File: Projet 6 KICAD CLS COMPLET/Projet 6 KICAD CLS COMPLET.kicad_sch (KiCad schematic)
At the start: 17 parts, among them J1 Conn_02x20_Odd_Even, J2 Conn_01x06, J3 Screw_Terminal_01x04, J4 Screw_Terminal_01x04, U2 AZ1117-3.3, U3 LSM6DSOX

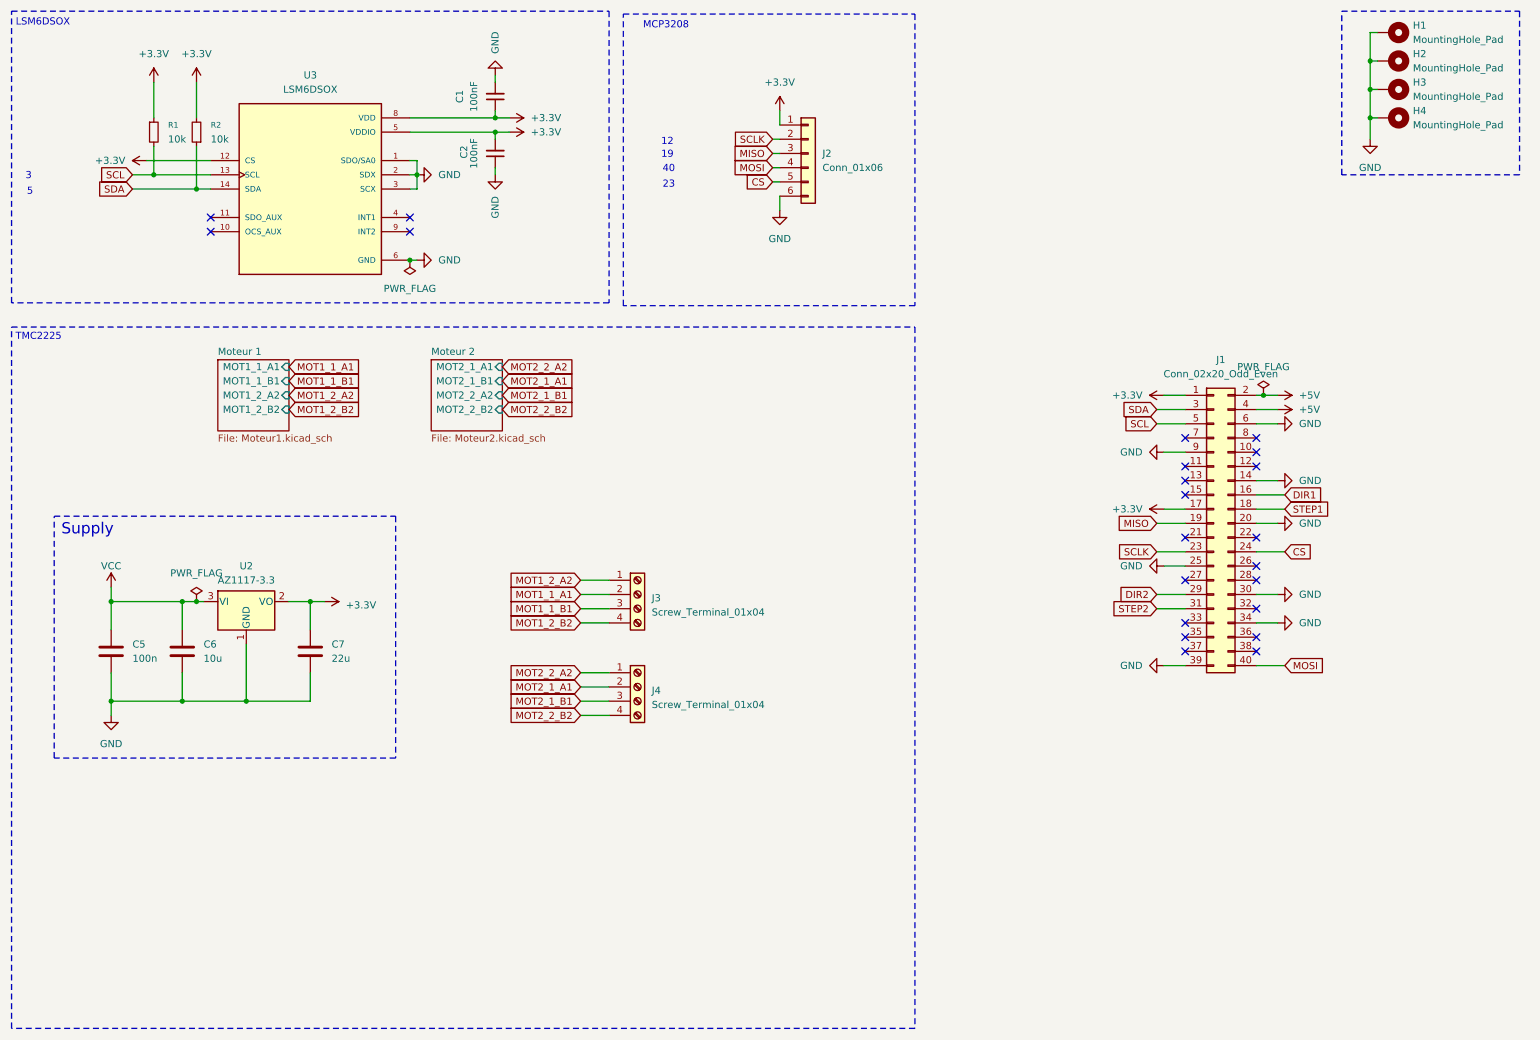
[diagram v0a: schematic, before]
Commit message: Projet 6 KICAD CLS COMPLET Correction
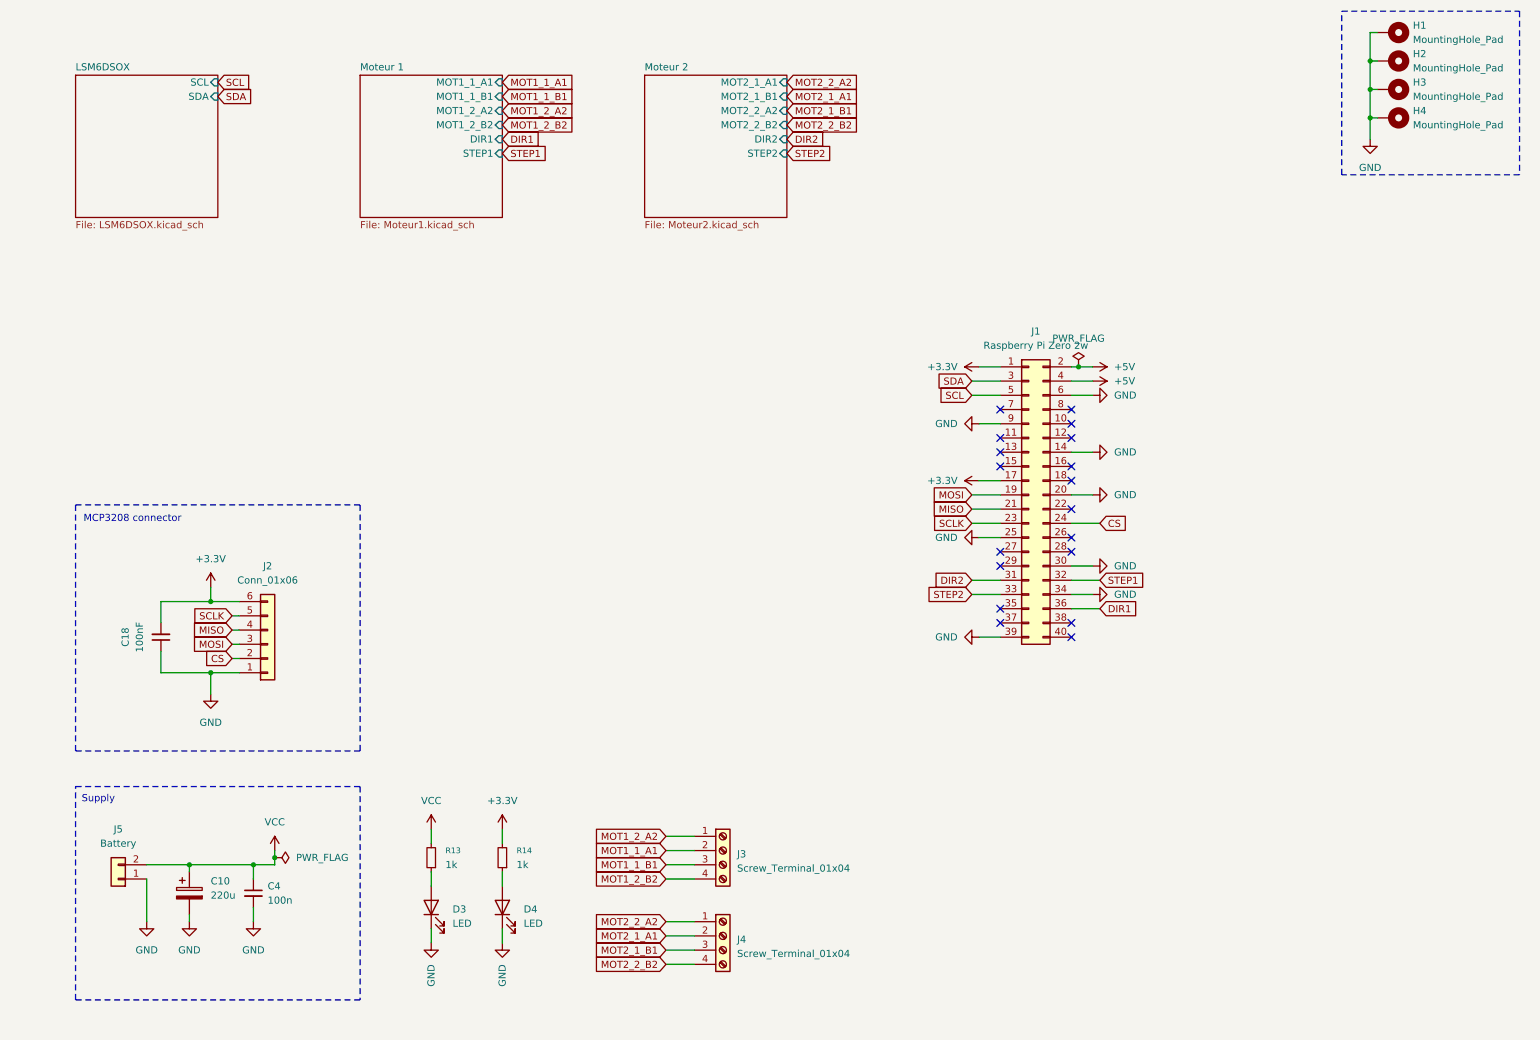
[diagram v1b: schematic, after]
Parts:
- removed C1, C2: 100nF, symbol Device:C_Small
- removed C5: 100n, symbol Device:C
- removed C6: 10u, symbol Device:C
- removed C7: 22u, symbol Device:C
- removed R1, R2: 10k, symbol Device:R_Small
- removed U2: AZ1117-3.3, symbol Regulator_Linear:AZ1117-3.3
- removed U3: LSM6DSOX, LSM6DSOX:PQFN50P250X300X86-14N, symbol LSM6DSOX:LSM6DSOX
- added C10: 220u, symbol Device:C_Polarized
- added C18: 100nF, symbol Device:C_Small
- added C4: 100n, symbol Device:C_Small
- added D3, D4: LED, symbol Device:LED
- added J5: Battery, symbol Connector_Generic:Conn_01x02
- added R13, R14: 1k, symbol Device:R_Small
- J1: value Conn_02x20_Odd_Even -> Raspberry Pi Zero 2w
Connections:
- net +3.3V: now also J2.6 (Pin_6), C18.2, R14.2; no longer J2.1 (Pin_1)
- net CS: now also J2.2 (Pin_2); no longer J2.5 (Pin_5)
- net DIR1: now also J1.36 (Pin_36); no longer J1.16 (Pin_16)
- net DIR2: now also J1.31 (Pin_31); no longer J1.29 (Pin_29)
- net GND: now also J2.1 (Pin_1), C10.2, C18.1, C4.2, D3.1 (K), D4.1 (K), J5.1 (Pin_1); no longer J2.6 (Pin_6)
- net MISO: now also J1.21 (Pin_21), J2.4 (Pin_4); no longer J1.19 (Pin_19), J2.3 (Pin_3)
- net MOSI: now also J1.19 (Pin_19), J2.3 (Pin_3); no longer J1.40 (Pin_40), J2.4 (Pin_4)
- net SCLK: now also J2.5 (Pin_5); no longer J2.2 (Pin_2)
- net STEP1: now also J1.32 (Pin_32); no longer J1.18 (Pin_18)
- net STEP2: now also J1.33 (Pin_33); no longer J1.31 (Pin_31)
- net VCC: now also C10.1, C4.1, J5.2 (Pin_2), R13.2
- new net: D4.2 (A), R14.1
- new net: D3.2 (A), R13.1
- no-connect marks 22 -> 18
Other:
- added sheet LSM6DSOX (LSM6DSOX.kicad_sch)
- sheet Moteur 1 ports: added DIR1, STEP1; removed none
- sheet Moteur 2 ports: added DIR2, STEP2; removed none
- note added: "MCP3208 connector"
- note removed: "12"
- note removed: "19"
- note removed: "23"
- note removed: "3"
- note removed: "40"
- note removed: "5"
- note removed: "LSM6DSOX"
- note removed: "MCP3208"
- note removed: "TMC2225"
- company: (none) -> ENSEA
- title: (none) -> Projet 6 PCB COMPLET
- moved on the sheet: J1, J2, J3, J4
